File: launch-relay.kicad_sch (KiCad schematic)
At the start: 0 parts

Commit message: started schematic
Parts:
- added U1: (no value), RF_Module:BM78SPPS5XC2, symbol HPRC_Sensors:BMA580
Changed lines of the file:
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@@
 	(generator_version "10.0")
 	(paper "A4")
+	(symbol
+		(lib_id "HPRC_Sensors:BMA580")
+		(at 48.26 167.64 0)
+		(unit 1)
+		(body_style 1)
+		(exclude_from_sim no)
+		(in_bom yes)
+		(on_board yes)
+		(in_pos_files yes)
+		(dnp no)
+		(fields_autoplaced yes)
+		(property "Reference" "U1"
+			(at 48.26 157.48 0)
+			(show_name no)
+			(do_not_autoplace no)
+			(effects
+				(font
+					(size 1.27 1.27)
+				)
+			)
+		)
+		(property "Value" ""
+			(at 48.26 167.64 0)
+			(show_name no)
+			(do_not_autoplace no)
+			(effects
+				(font
+					(size 1.27 1.27)
+				)
+			)
+		)
+		(property "Footprint" "RF_Module:BM78SPPS5XC2"
+			(at 48.26 167.64 0)
+			(hide yes)
+			(show_name no)
+			(do_not_autoplace no)
+			(effects
+				(font
+					(size 1.27 1.27)
+				)
+			)
+		)
+		(property "Datasheet" ""
+			(at 48.26 167.64 0)
+			(hide yes)
+			(show_name no)
+			(do_not_autoplace no)
+			(effects
+				(font
+					(size 1.27 1.27)
+				)
+			)
+		)
+		(property "Description" ""
+			(at 48.26 167.64 0)
+			(hide yes)
+			(show_name no)
+			(do_not_autoplace no)
+			(effects
+				(font
+					(size 1.27 1.27)
+				)
+			)
+		)
+		(pin "1"
+		)
+		(pin "6"
+		)
+		(pin "4"
+		)
+		(pin "3"
+		)
+		(pin "2"
+		)
+		(pin "5"
+		)
+		(instances
+			(project "launch-relay"
+				(path "/5fd10500-b703-4d79-824f-0c6e126f5ac0"
+					(reference "U1")
+					(unit 1)
+				)
+			)
+		)
+	)
 	(sheet_instances
 		(path "/"

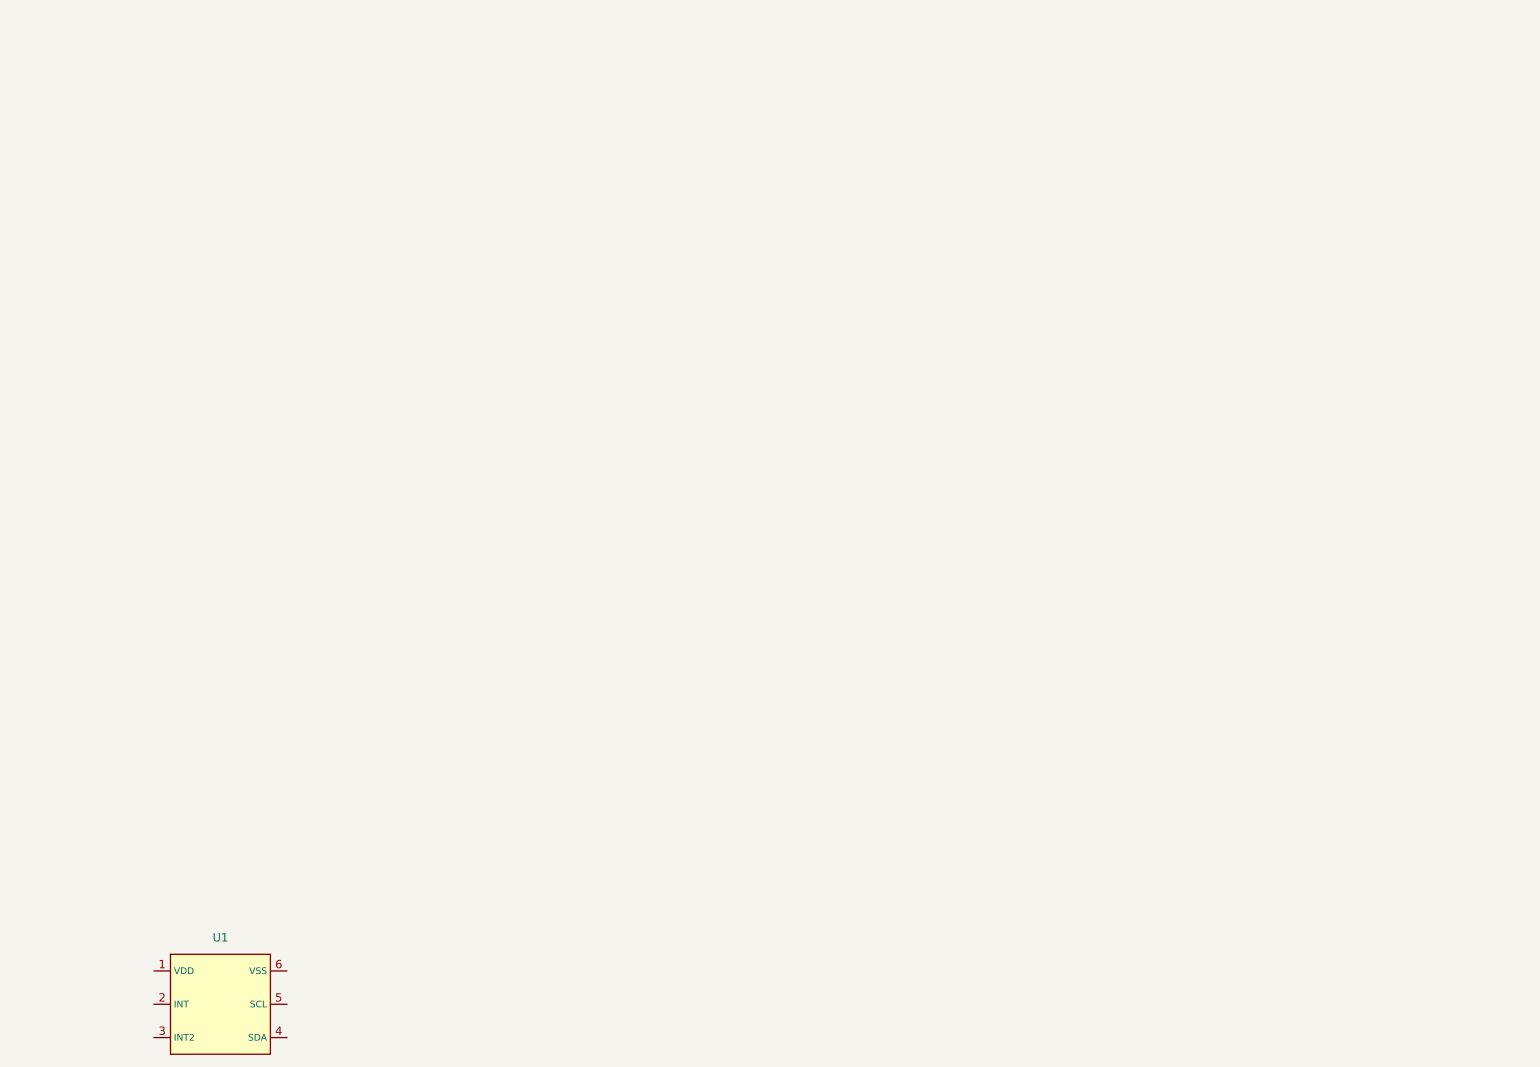
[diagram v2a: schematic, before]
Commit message: started schematic
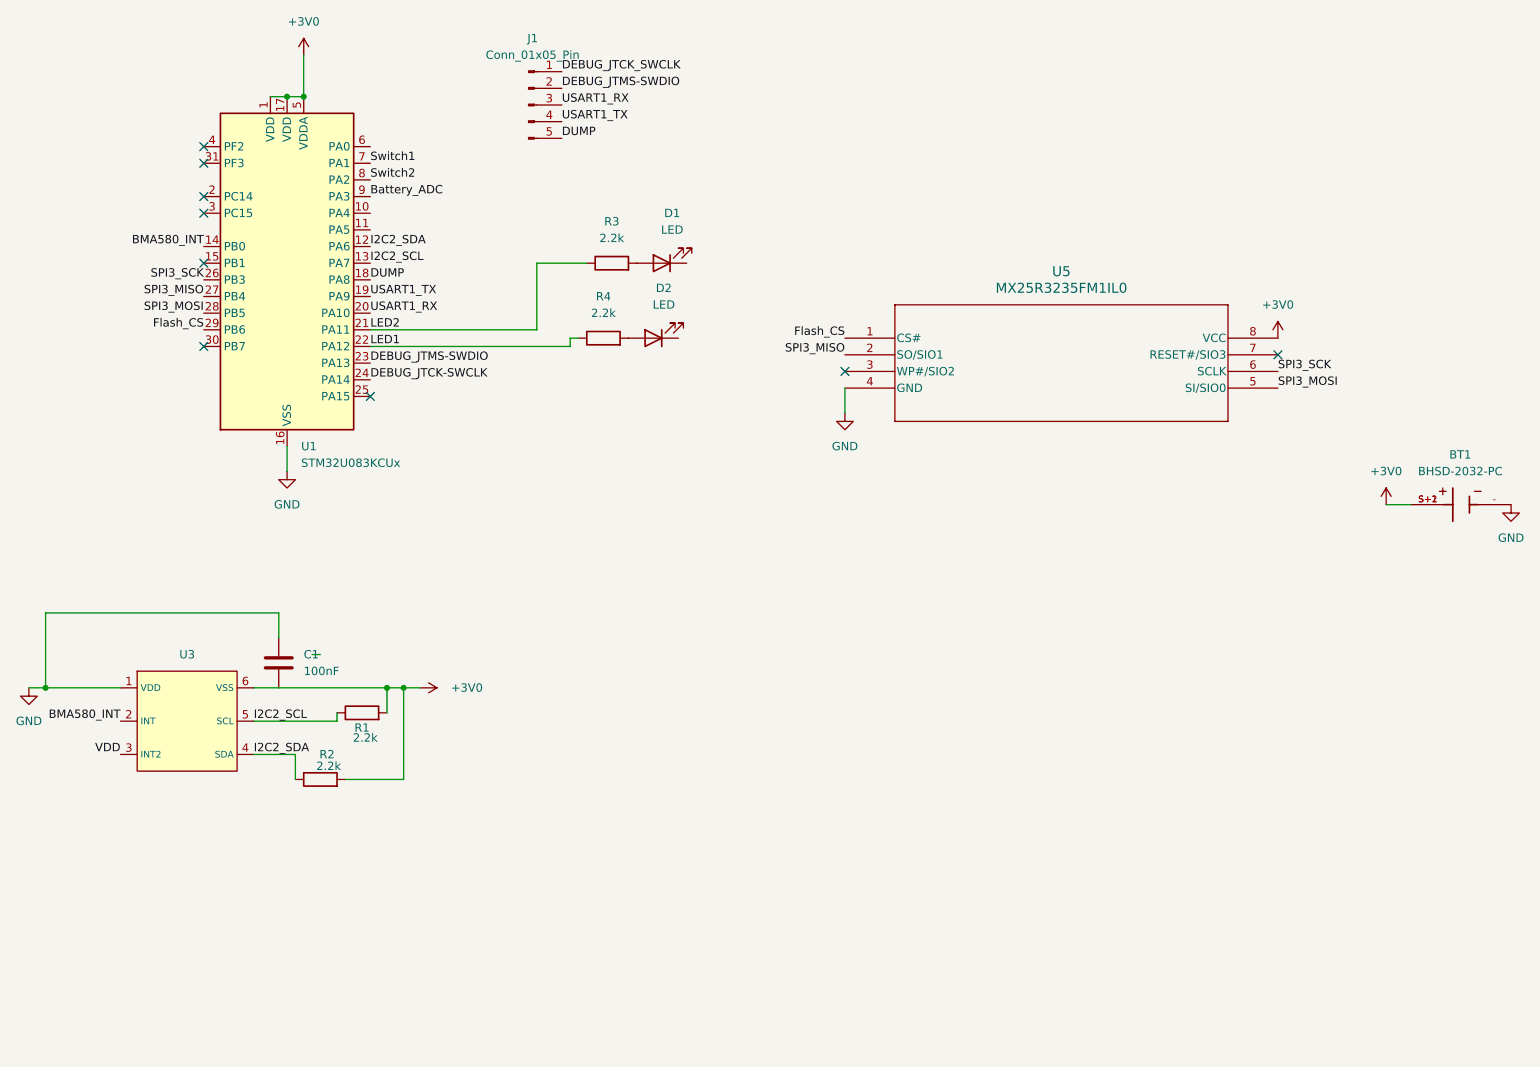
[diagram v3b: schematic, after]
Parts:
- removed U1: (no value), RF_Module:BM78SPPS5XC2, symbol HPRC_Sensors:BMA580
- added BT1: BHSD-2032-PC, BHSD-2032-PC:BAT_BHSD-2032-PC, symbol BHSD-2032-PC:BHSD-2032-PC
- added C1: 100nF, symbol Device:C
- added D1, D2: LED, symbol Device:LED
- added J1: Conn_01x05_Pin, Package_DFN_QFN:QFN-20-1EP_5x5mm_P0.65mm_EP3.35x3.35mm, symbol Connector:Conn_01x05_Pin
- added R1, R2, R3, R4: 2.2k, symbol Device:R
- added U1: STM32U083KCUx, Package_DFN_QFN:QFN-32-1EP_5x5mm_P0.5mm_EP3.45x3.45mm, symbol MCU_ST_STM32U0:STM32U083KCUx
- added U3: (no value), RF_Module:BM78SPPS5XC2, symbol HPRC_Sensors:BMA580
- added U5: MX25R3235FM1IL0, SOP_8L_150_MAC, symbol MX25R3235FM1IL0:MX25R3235FM1IL0
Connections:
- new net: D1.2 (A), R3.2
- new net: D2.2 (A), R4.2
- new net +3V0: BT1.S+1, BT1.S+2, R1.2, R2.2, U1.1 (VDD), U1.17 (VDD), U1.5 (VDDA), U3.6 (VSS), U5.8 (VCC)
- new net BMA580_INT: U1.14 (PB0), U3.2 (INT)
- new net Battery_ADC: U1.9 (PA3)
- new net DEBUG_JTCK-SWCLK: U1.24 (PA14)
- new net DEBUG_JTCK_SWCLK: J1.1 (Pin_1)
- new net DEBUG_JTMS-SWDIO: J1.2 (Pin_2), U1.23 (PA13)
- new net DUMP: J1.5 (Pin_5), U1.18 (PA8)
- new net Flash_CS: U1.29 (PB6), U5.1 (CS#)
- new net GND: BT1.-, C1.1, U1.16 (VSS), U1.32 (VSS), U1.33 (VSS), U3.1 (VDD), U5.4 (GND)
- new net I2C2_SCL: R1.1, U1.13 (PA7), U3.5 (SCL)
- new net I2C2_SDA: R2.1, U1.12 (PA6), U3.4 (SDA)
- new net LED1: R4.1, U1.22 (PA12)
- new net LED2: R3.1, U1.21 (PA11)
- new net SPI3_MISO: U1.27 (PB4), U5.2 (SO/SIO1)
- new net SPI3_MOSI: U1.28 (PB5), U5.5 (SI/SIO0)
- new net SPI3_SCK: U1.26 (PB3), U5.6 (SCLK)
- new net Switch1: U1.7 (PA1)
- new net Switch2: U1.8 (PA2)
- new net USART1_RX: J1.3 (Pin_3), U1.20 (PA10)
- new net USART1_TX: J1.4 (Pin_4), U1.19 (PA9)
- new net VDD: U3.3 (INT2)
- no-connect marks 0 -> 9
